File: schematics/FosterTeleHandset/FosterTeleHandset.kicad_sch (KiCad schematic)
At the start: 7 parts, among them Q1 2N2222, U1 US1881EUA-AAA-000-BU, U2 RASPBERRY_PI_PICO

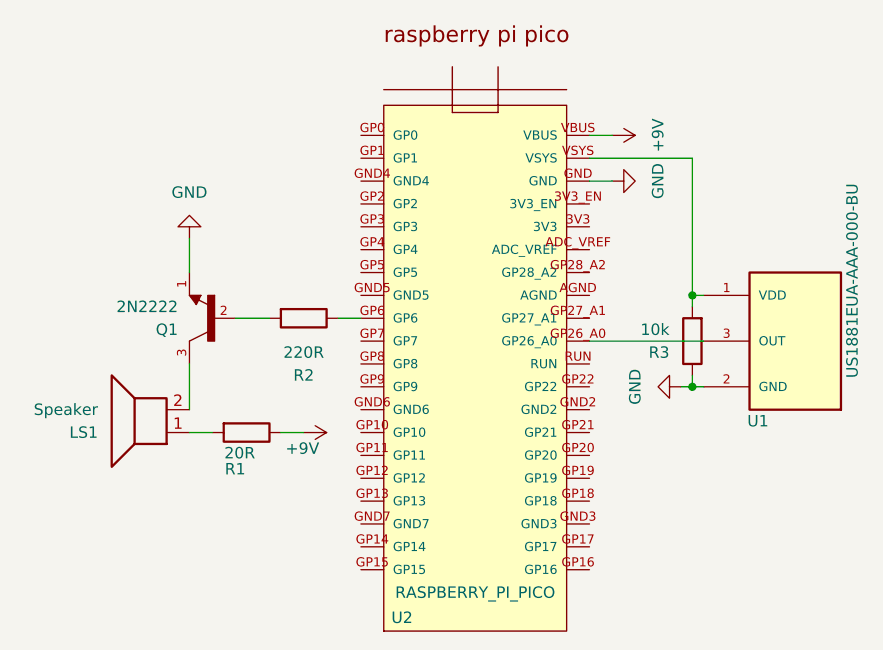
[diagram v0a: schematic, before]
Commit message: Adjusted schematic.
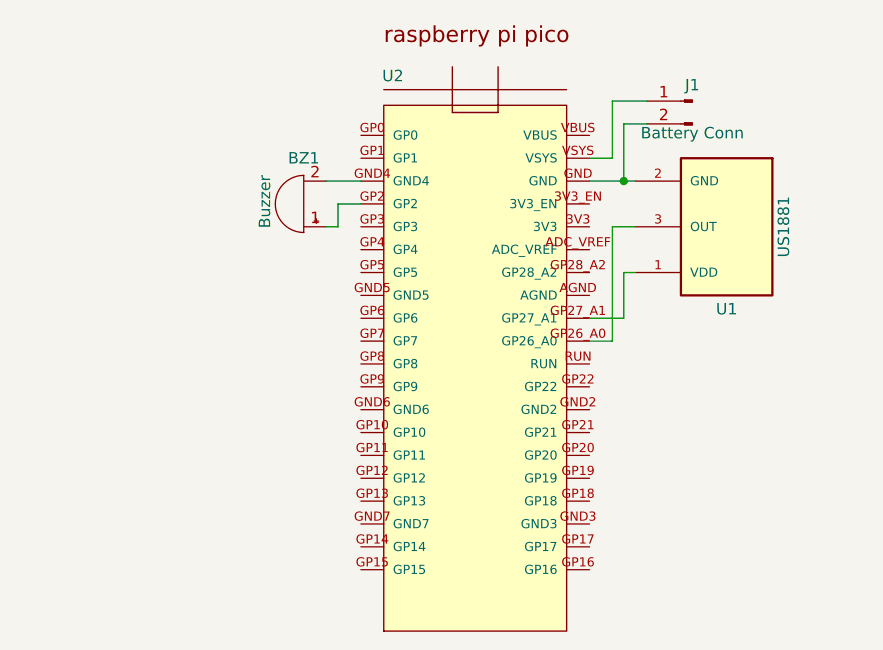
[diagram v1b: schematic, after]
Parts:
- removed LS1: Speaker, symbol Device:Speaker
- removed Q1: 2N2222, 2N2222:TO127P584H533-3, symbol 2N2222:2N2222
- removed R1: 20R, symbol Device:R
- removed R2: 220R, symbol Device:R
- removed R3: 10k, symbol Device:R
- added BZ1: Buzzer, symbol Device:Buzzer
- added J1: Battery Conn, symbol Connector:Conn_01x02_Pin
- U1: value US1881EUA-AAA-000-BU -> US1881
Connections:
- net at U1.1 (VDD): now also U2.GP27_A1; no longer U2.VSYS
- net at U2.GND4: now also BZ1.2 (-)
- net at U2.GP2: now also BZ1.1 (+)
- net +9V: no longer names the net of U2.VBUS
- net GND: no longer names the net of U1.2 (GND), U2.GND
- net GND: now also J1.2 (Pin_2)
- new net: J1.1 (Pin_1), U2.VSYS
